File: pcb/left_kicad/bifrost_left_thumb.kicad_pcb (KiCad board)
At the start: 2 copper layers, 58.5 x 21 mm, 12 parts, among them J1 Conn_01x06, SW1 1U, SW2 1U, SW3 1U

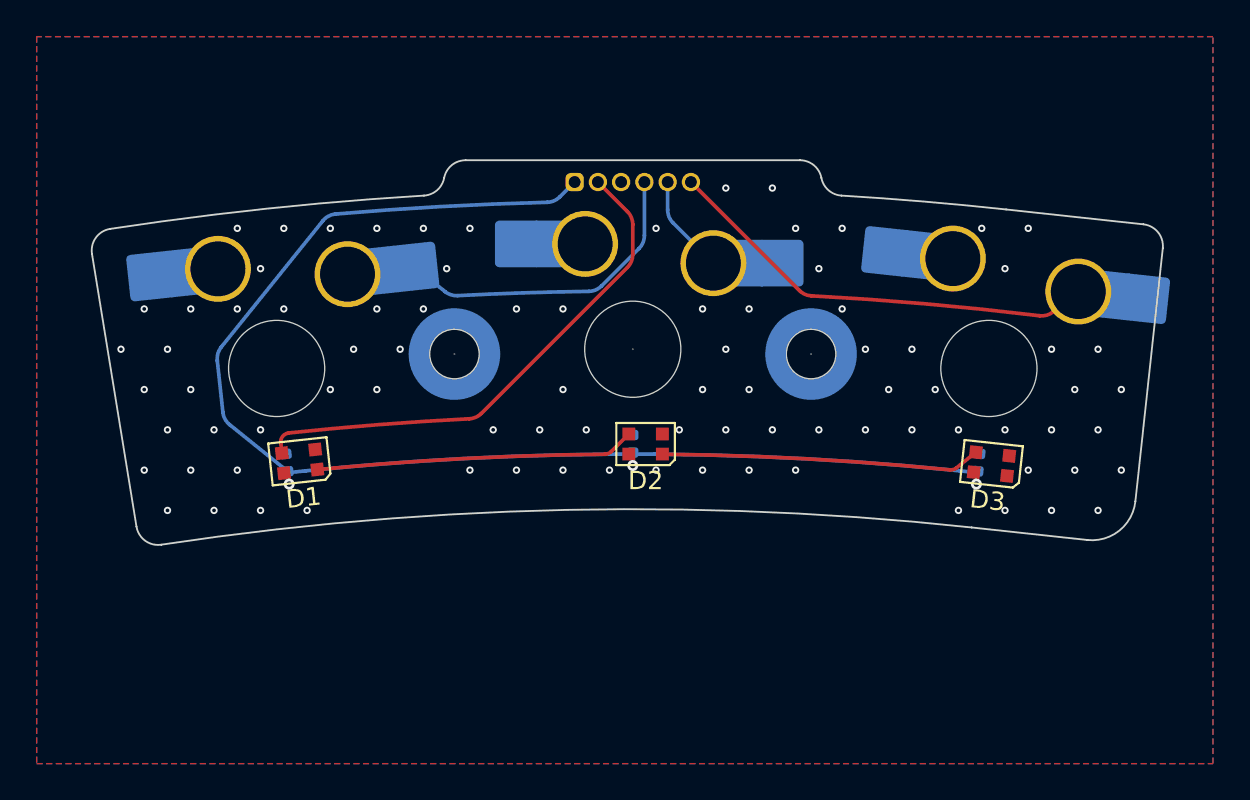
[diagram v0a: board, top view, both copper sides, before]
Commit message: Update PCB designs and fabrication outputs
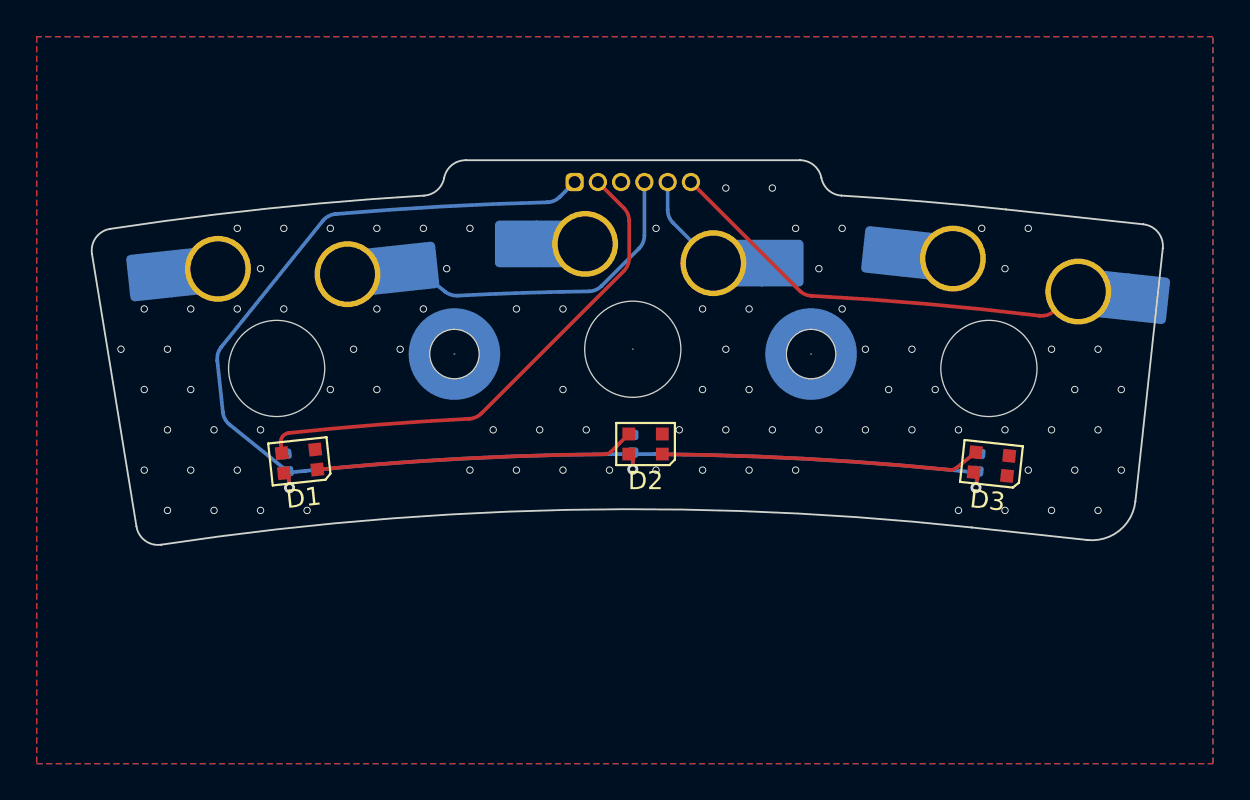
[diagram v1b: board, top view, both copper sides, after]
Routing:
- net RGB_PWR: track 73.7 -> 74.9 mm
